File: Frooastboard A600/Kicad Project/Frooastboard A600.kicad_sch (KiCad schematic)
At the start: 204 parts, among them J1 PS2_5V, J3 SW Interface, J8 USB, Q1 BSS138, Q2 BSS138, U2 RP2040, U3 W25Q32JVZP, U4 LM317L_SOT-89, Y1 12MHz

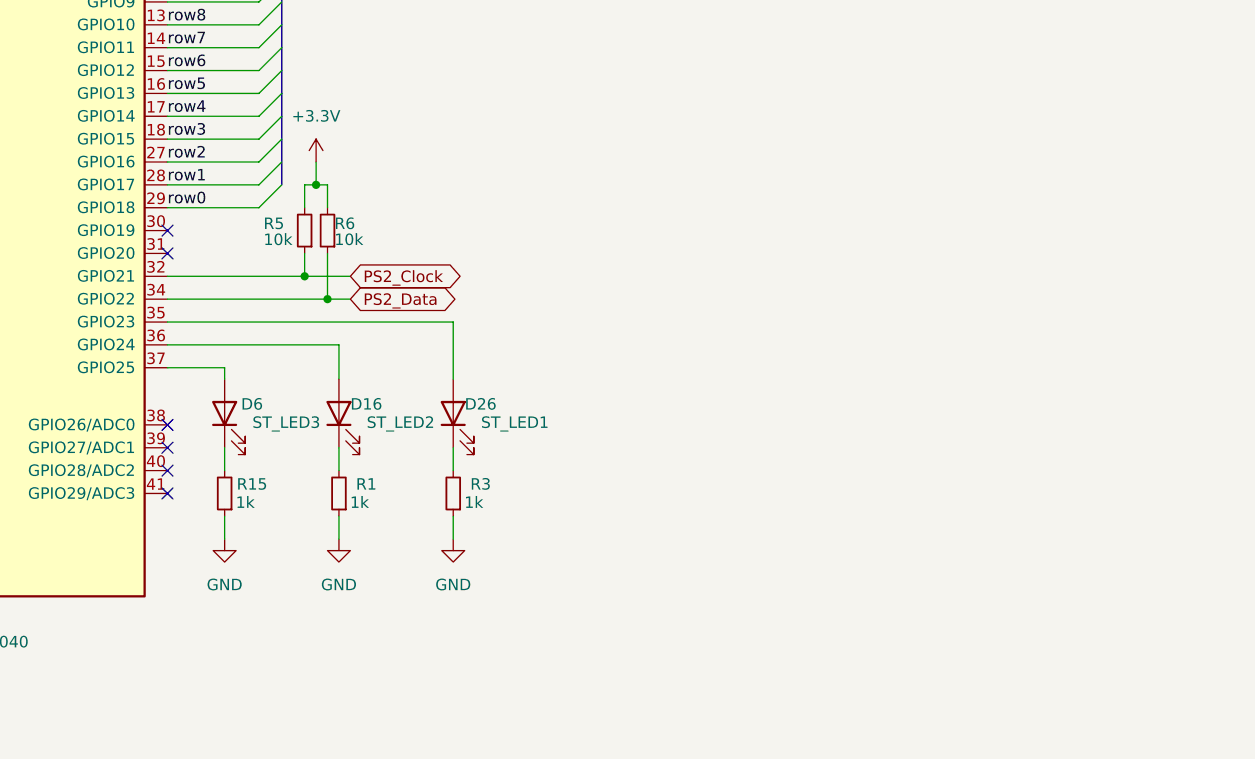
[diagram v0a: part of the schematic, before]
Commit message: more led stuff NOT REVERSED YET
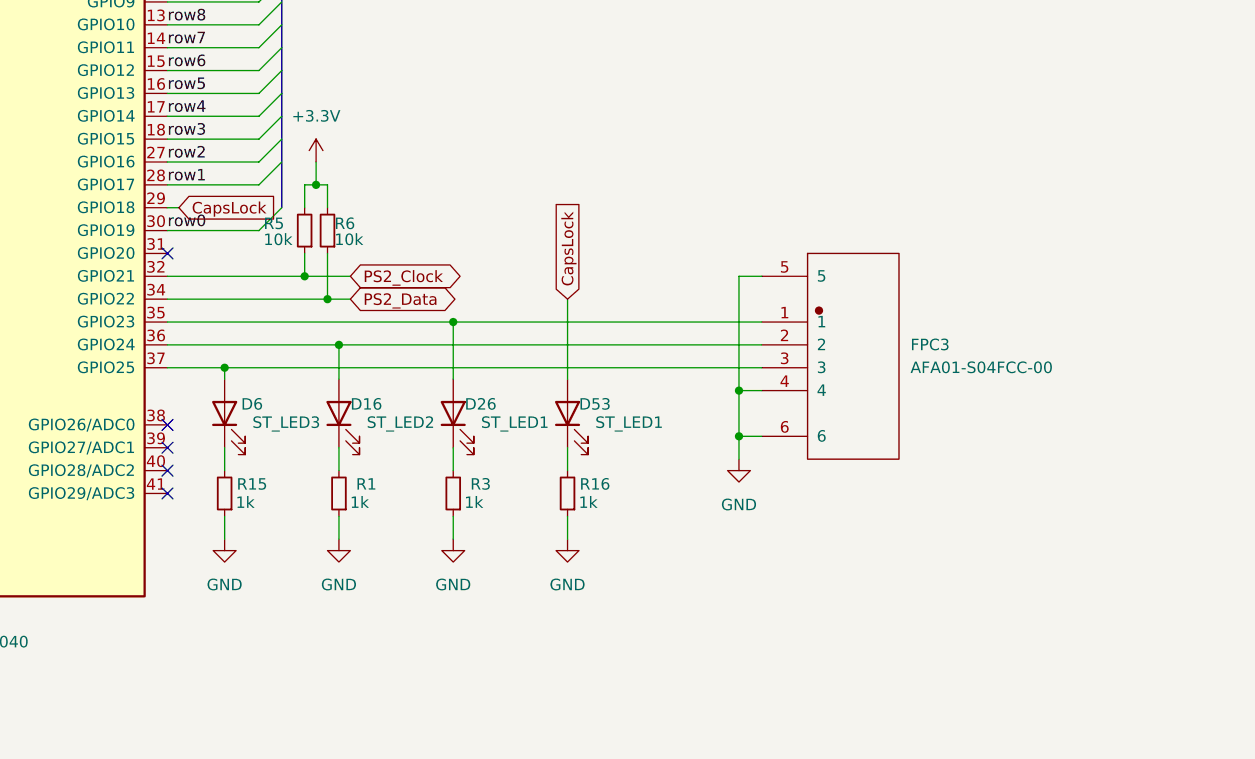
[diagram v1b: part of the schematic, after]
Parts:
- added D53: ST_LED1, LED_SMD:LED_PLCC-2_3.4x3.0mm_KA, symbol Device:LED
- added FPC3: AFA01-S04FCC-00, AFA01-SXXFCX-00:FPC-SMD_4P-P1.00_AFA01-S04FCC-00, symbol AFA01-SXXFCX-00:AFA01-S04FCC-00
- added R16: 1k, Resistor_SMD:R_0805_2012Metric, symbol Device:R_Small
- MX1: footprint MX_Hotswap:MX-Hotswap-1.5U -> MX_Solderable:MX-Solderable-1.5U
- MX10, MX15, MX19, MX21, MX26, MX32, MX37, MX4, MX41, MX42, MX48, MX55, MX6, MX60, MX67, MX8: footprint MX_Hotswap:MX-Hotswap-1.25U -> MX_Solderable:MX-Solderable-1.25U
- MX11, MX12, MX13, MX14, MX16, MX17, MX18, MX2, MX22, MX23, MX24, MX25, MX27, MX28, MX29, MX3, MX33, MX34, MX35, MX36, MX38, MX39, MX40, MX43, MX44, MX45, MX46, MX47, MX49, MX50, MX51, MX52, MX53, MX54, MX56, MX57, MX59, MX61, MX62, MX63, MX65, MX66, MX69, MX71, MX72, MX73, MX74, MX75, MX76, MX78, MX81, MX87, MX88, MX89, MX90, MX94: footprint MX_Hotswap:MX-Hotswap-1U -> MX_Solderable:MX-Solderable-1U
- MX30: footprint MX_Hotswap:MX-Hotswap-8U -> MX_Solderable:MX-Solderable-8U
- MX5: footprint MX_Hotswap:MX-Hotswap-2U -> MX_Solderable:MX-Solderable-2U
- MX58, MX7: footprint MX_Hotswap:MX-Hotswap-1.75U -> MX_Solderable:MX-Solderable-1.75U
- MX68: footprint MX_Hotswap:MX-Hotswap-ISO -> MX_Solderable:MX-Solderable-ISO
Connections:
- net GND: now also FPC3.4, FPC3.5, FPC3.6, R16.1
- net row0: now also U2.30 (GPIO19); no longer U2.29 (GPIO18)
- net at D26.2 (A), U2.35 (GPIO23): now also FPC3.1
- net at D16.2 (A), U2.36 (GPIO24): now also FPC3.2
- net at D6.2 (A), U2.37 (GPIO25): now also FPC3.3
- new net: D53.1 (K), R16.2
- new net CapsLock: D53.2 (A), U2.29 (GPIO18)
- no-connect marks 8 -> 7

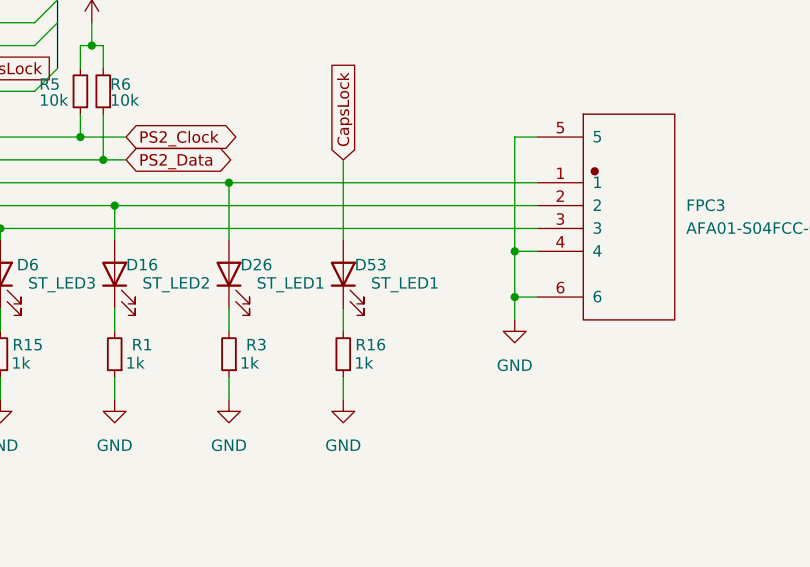
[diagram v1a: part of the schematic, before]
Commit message: new leds (finally)
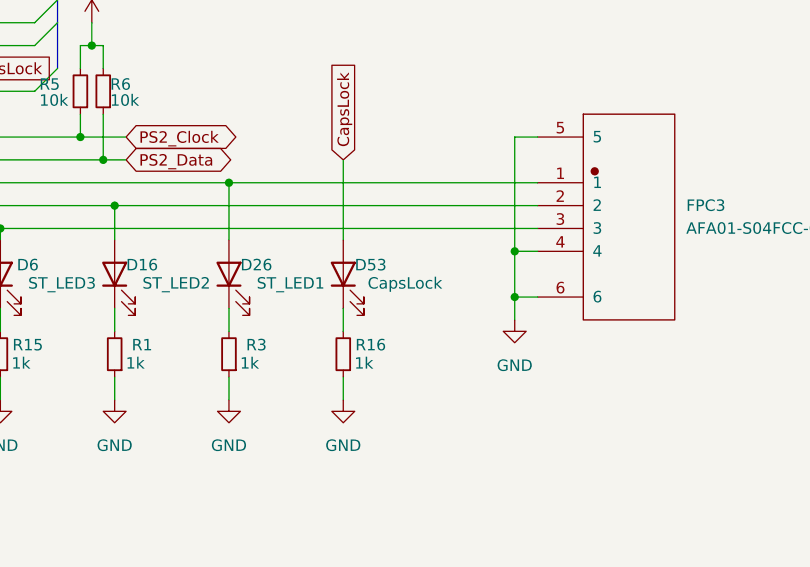
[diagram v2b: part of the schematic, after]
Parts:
- D16, D26, D6: footprint LED_SMD:LED_PLCC-2_3.4x3.0mm_KA -> Frooastboard Footprints:LED_RGB_SMD_6028_Reverse
- D53: value ST_LED1 -> CapsLock; footprint LED_SMD:LED_PLCC-2_3.4x3.0mm_KA -> Frooastboard Footprints:LED_RGB_SMD_6028_Reverse
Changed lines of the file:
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@@
 			)
 		)
-		(property "Value" "ST_LED1"
+		(property "Value" "CapsLock"
 			(at 159.258 114.046 90)
 			(effects
@@
 			)
 		)
-		(property "Footprint" "LED_SMD:LED_PLCC-2_3.4x3.0mm_KA"
+		(property "Footprint" "Frooastboard Footprints:LED_RGB_SMD_6028_Reverse"
 			(at 152.4 113.03 0)
 			(effects
@@
 			)
 		)
-		(property "Footprint" "LED_SMD:LED_PLCC-2_3.4x3.0mm_KA"
+		(property "Footprint" "Frooastboard Footprints:LED_RGB_SMD_6028_Reverse"
 			(at 139.7 113.03 0)
 			(effects
@@
 			)
 		)
-		(property "Footprint" "LED_SMD:LED_PLCC-2_3.4x3.0mm_KA"
+		(property "Footprint" "Frooastboard Footprints:LED_RGB_SMD_6028_Reverse"
 			(at 114.3 113.03 0)
 			(effects
@@
 			)
 		)
-		(property "Footprint" "LED_SMD:LED_PLCC-2_3.4x3.0mm_KA"
+		(property "Footprint" "Frooastboard Footprints:LED_RGB_SMD_6028_Reverse"
 			(at 127 113.03 0)
 			(effects

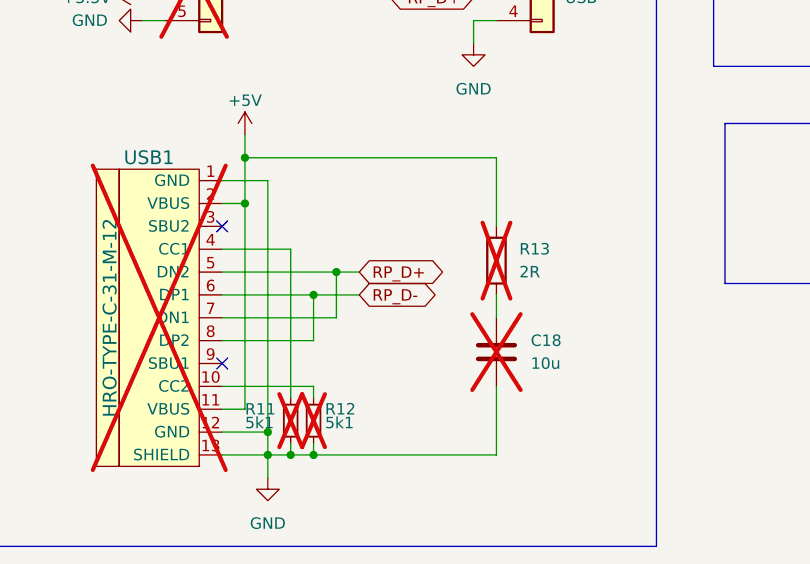
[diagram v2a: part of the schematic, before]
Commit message: bug fixes
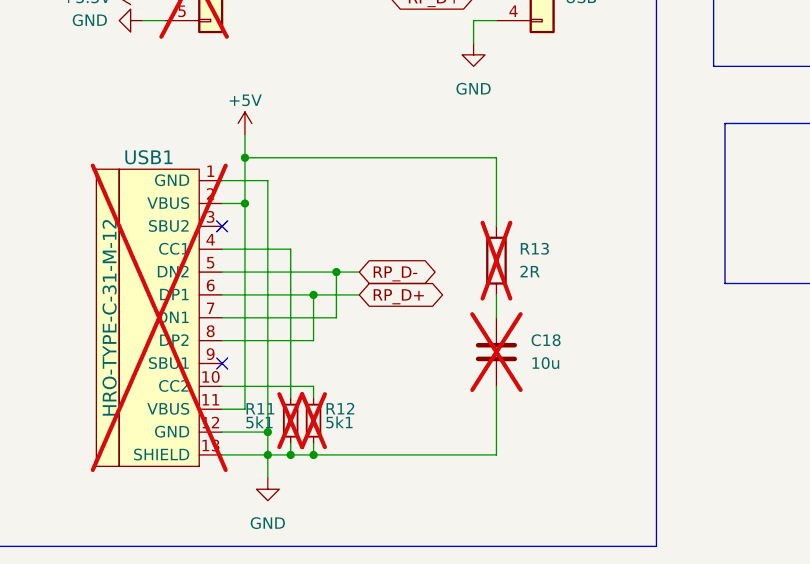
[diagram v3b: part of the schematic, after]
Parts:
- MX30: footprint MX_Solderable:MX-Solderable-8U -> MX_Solderable:MX-Solderable-7U
- MX52: footprint MX_Solderable:MX-Solderable-1U -> MX_Solderable:MX-Solderable-1.25U
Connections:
- net RP_D+: now also USB1.6 (DP1), USB1.8 (DP2); no longer USB1.5 (DN2), USB1.7 (DN1)
- net RP_D-: now also USB1.5 (DN2), USB1.7 (DN1); no longer USB1.6 (DP1), USB1.8 (DP2)
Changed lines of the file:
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@@
 	(global_label "RP_D+"
 		(shape bidirectional)
-		(at 238.76 246.38 0)
+		(at 238.76 248.92 0)
 		(fields_autoplaced yes)
 		(effects
@@
 		)
 		(property "Intersheetrefs" "${INTERSHEET_REFS}"
-			(at 249.2065 246.38 0)
+			(at 249.2065 248.92 0)
 			(effects
 				(font
@@
 	(global_label "RP_D-"
 		(shape bidirectional)
-		(at 238.76 248.92 0)
+		(at 238.76 246.38 0)
 		(fields_autoplaced yes)
 		(effects
@@
 		)
 		(property "Intersheetrefs" "${INTERSHEET_REFS}"
-			(at 249.2065 248.92 0)
+			(at 249.2065 246.38 0)
 			(effects
 				(font
@@
 			)
 		)
-		(property "Footprint" "MX_Solderable:MX-Solderable-1U"
+		(property "Footprint" "MX_Solderable:MX-Solderable-1.25U"
 			(at 320.04 132.08 90)
 			(effects
@@
 			)
 		)
-		(property "Footprint" "MX_Solderable:MX-Solderable-8U"
+		(property "Footprint" "MX_Solderable:MX-Solderable-7U"
 			(at 281.94 132.08 90)
 			(effects
